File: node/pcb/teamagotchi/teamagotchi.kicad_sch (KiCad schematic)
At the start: 2 parts

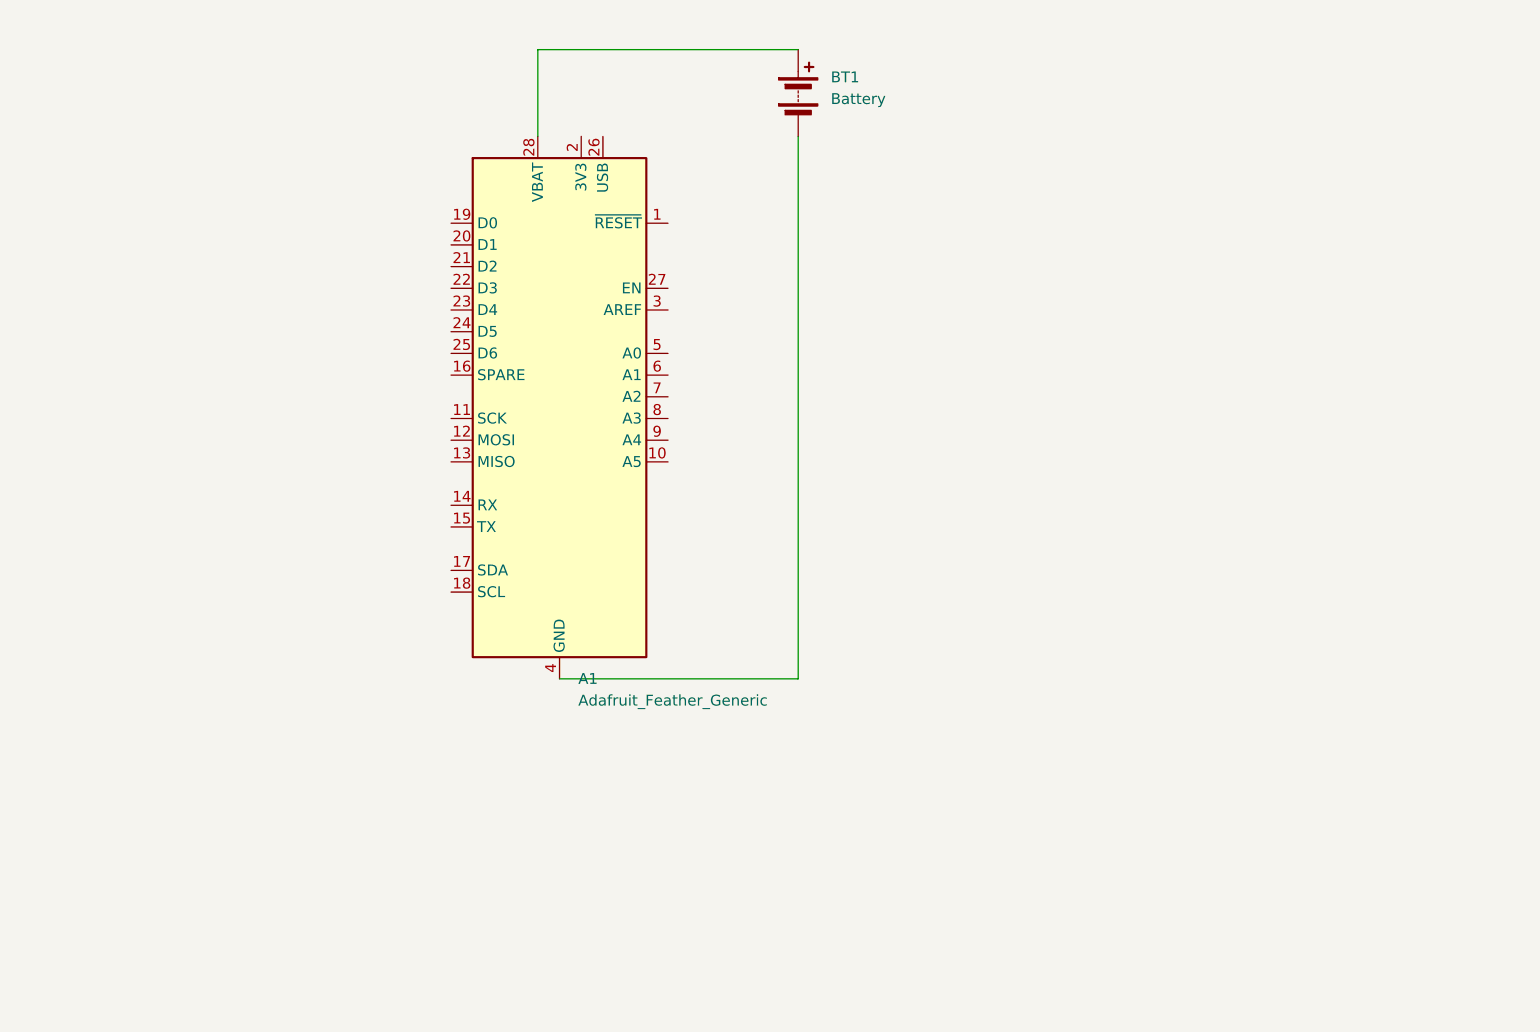
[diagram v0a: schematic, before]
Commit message: first shot of the pcv
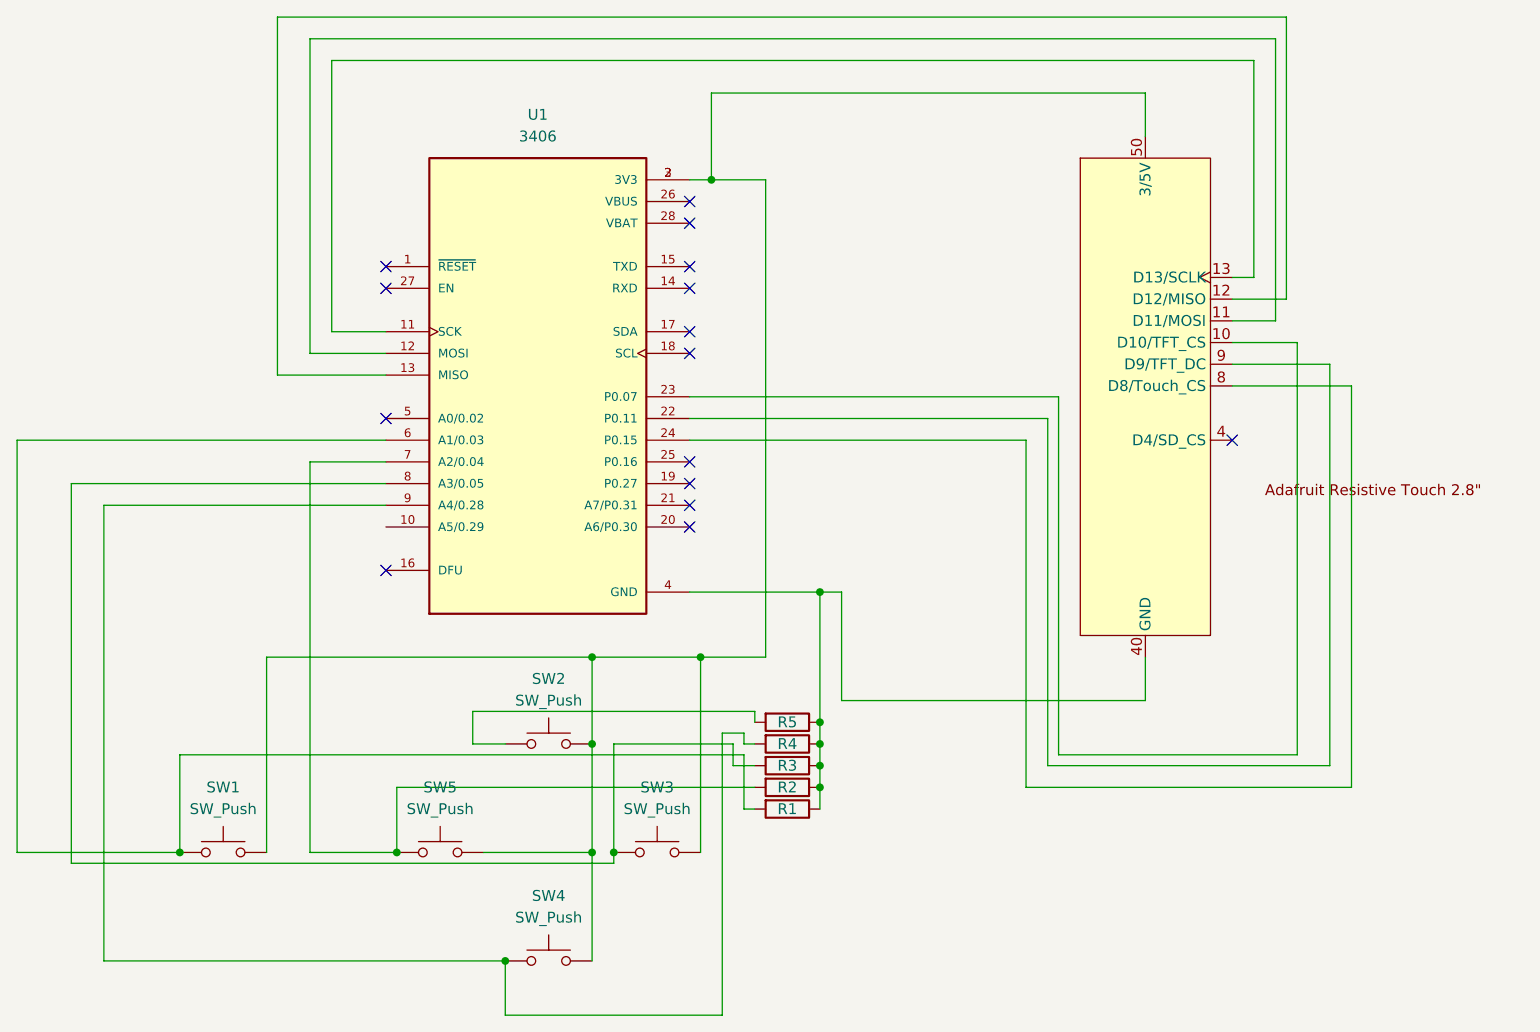
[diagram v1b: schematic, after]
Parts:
- removed A1: Adafruit_Feather_Generic, Module:Adafruit_Feather, symbol MCU_Module:Adafruit_Feather_Generic
- removed BT1: Battery, Battery:BatteryHolder_Keystone_103_1x20mm, symbol Device:Battery
- added R1, R2, R3, R4, R5: R, Resistor_THT:R_Axial_DIN0204_L3.6mm_D1.6mm_P7.62mm_Horizontal, symbol Device:R
- added SW1, SW2, SW3, SW4, SW5: SW_Push, Button_Switch_THT:SW_SPST_Omron_B3F-40xx, symbol Switch:SW_Push
- added TFT1: ~, Library:Display-2.8, symbol dispaly:display-2.8{dblquote}
- added U1: 3406, Library:MODULE_3406, symbol 3406:3406
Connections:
- new net: R1.2, SW1.1, U1.6 (A1/0.03)
- new net: SW1.2, SW2.2, SW3.2, SW4.2, SW5.2, TFT1.50 (3/5V), U1.2 (3V3), U1.3 (3V3)
- new net: R1.1, R2.1, R3.1, R4.1, R5.1, TFT1.40 (GND), U1.4 (GND)
- new net: R4.2, SW4.1, U1.9 (A4/0.28)
- new net: TFT1.10 (D10/TFT_CS), U1.23 (P0.07)
- new net: TFT1.11 (D11/MOSI), U1.12 (MOSI)
- new net: TFT1.12 (D12/MISO), U1.13 (MISO)
- new net: TFT1.13 (D13/SCLK), U1.11 (SCK)
- new net: TFT1.8 (D8/Touch_CS), U1.24 (P0.15)
- new net: TFT1.9 (D9/TFT_DC), U1.22 (P0.11)
- new net: R3.2, SW3.1, U1.8 (A3/0.05)
- new net: R5.2, SW2.1
- new net: R2.2, SW5.1, U1.7 (A2/0.04)
- no-connect marks 0 -> 15
